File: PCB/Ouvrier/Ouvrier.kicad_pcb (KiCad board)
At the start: 2 copper layers, 7 parts, among them Q1 2N2220, U1 XIAO-ESP32-S3-Plus-DIP, U2 BMP581, U3 UWB

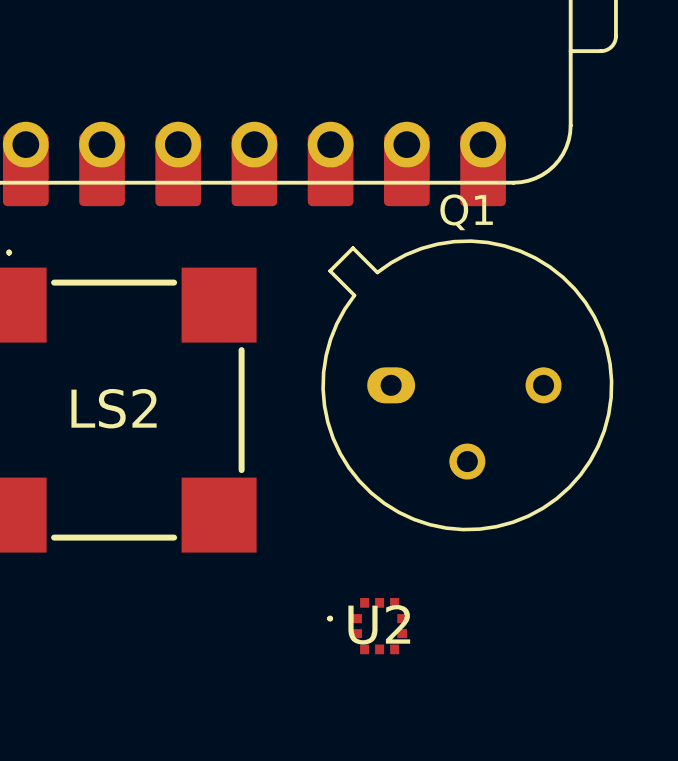
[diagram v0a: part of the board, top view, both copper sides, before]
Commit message: MaJ batterie KiCad Ouvrier
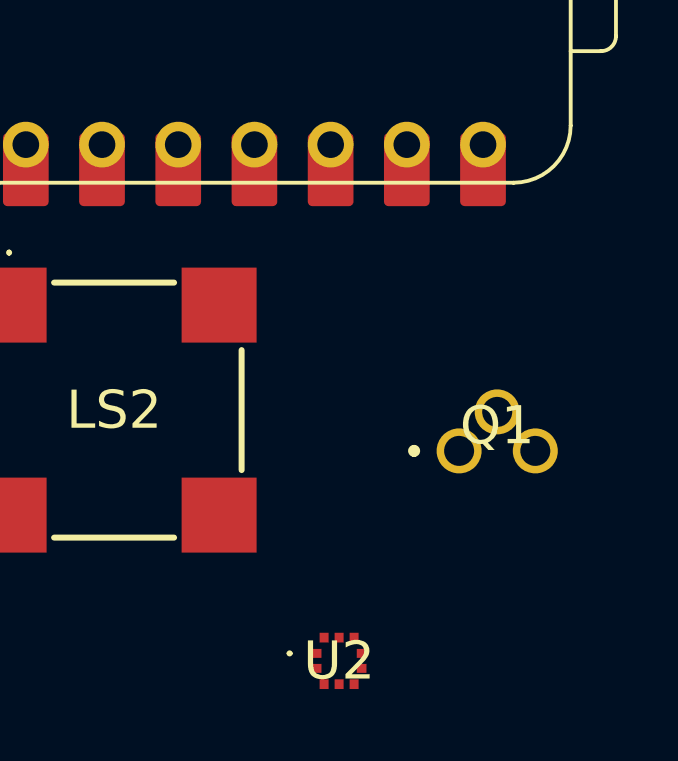
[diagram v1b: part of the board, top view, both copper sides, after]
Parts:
- Q1: value 2N2220 -> 2N2222B; footprint Package_TO_SOT_THT:TO-39-3 -> Bibliotheque_Projet:2N2222B
- moved Q1 3.15 mm to (149.5, 96.5)
- moved U2 1.78 mm to (145.5, 103.5)
